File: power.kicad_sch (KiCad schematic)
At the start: 32 parts, among them J18 Conn_01x06, U32 LTC4121, U33 BQ25883RGER

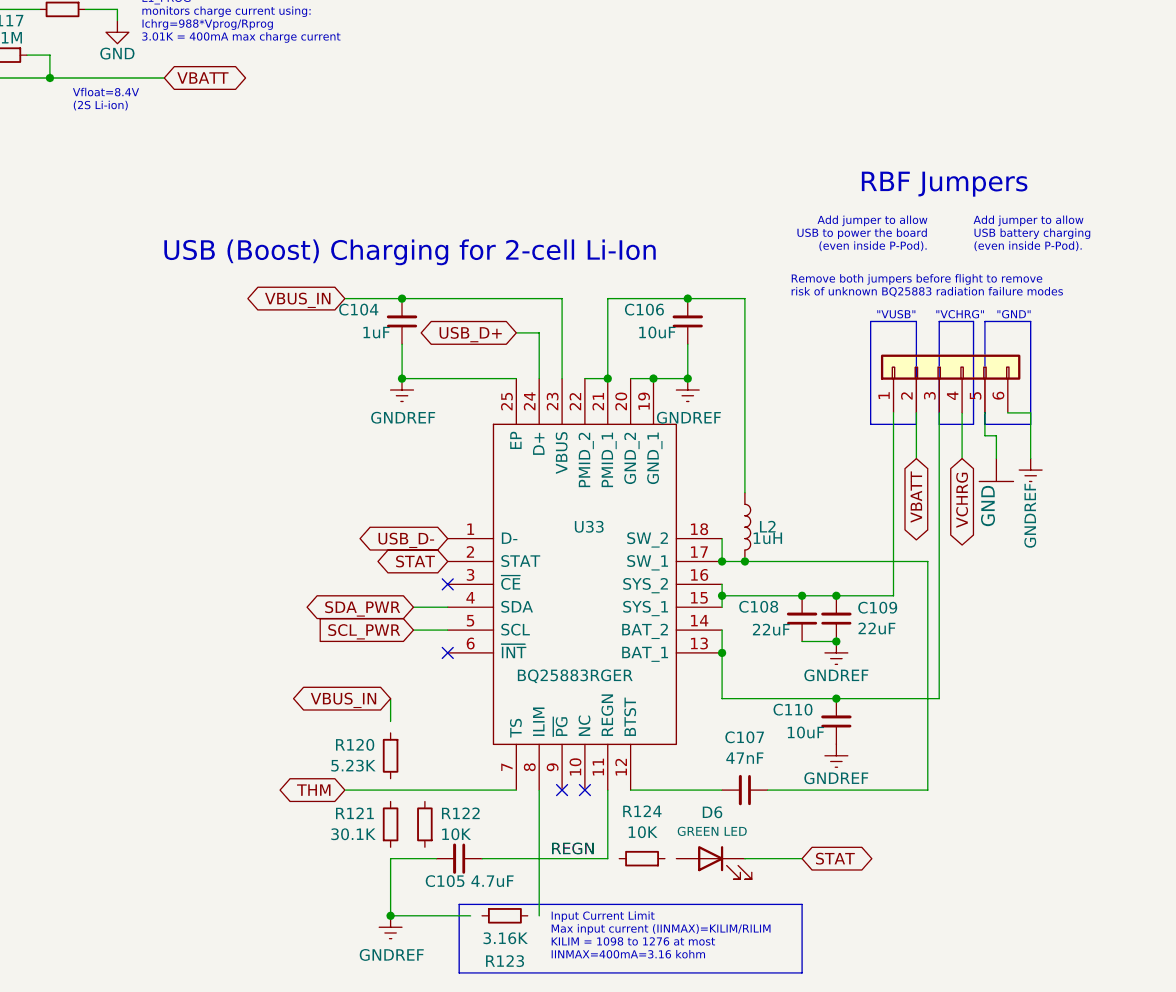
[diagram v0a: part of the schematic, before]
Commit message: Backup
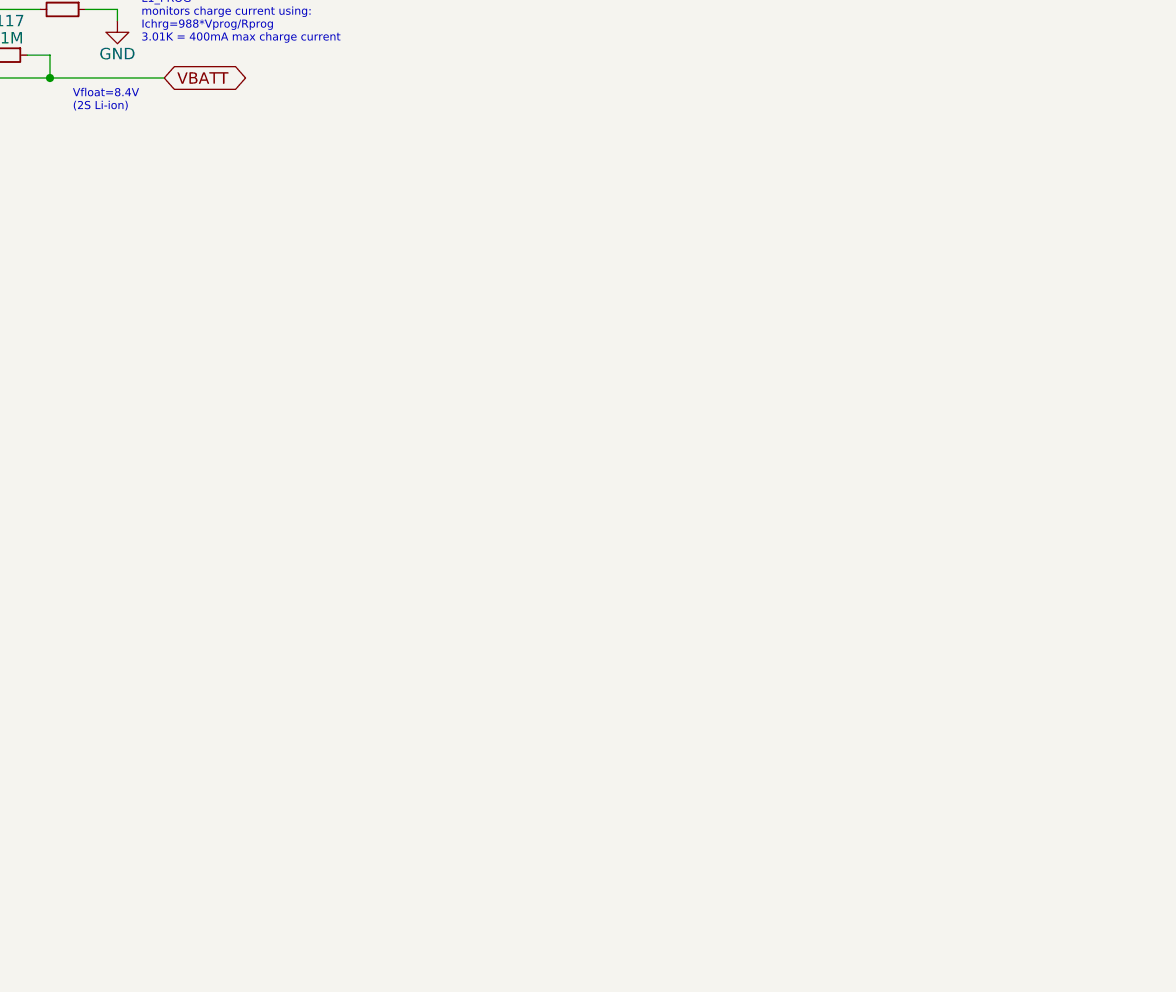
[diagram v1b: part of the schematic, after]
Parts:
- removed C104: 1uF, Capacitor_SMD:C_0603_1608Metric, symbol Device:C_Small
- removed C105: 4.7uF, Capacitor_SMD:C_0603_1608Metric, symbol Device:C_Small
- removed C106, C110: 10uF, Capacitor_SMD:C_0603_1608Metric, symbol Device:C_Small
- removed C107: 47nF, Capacitor_SMD:C_0603_1608Metric, symbol Device:C_Small
- removed C108, C109: 22uF, Capacitor_SMD:C_0603_1608Metric, symbol Device:C_Small
- removed D6: GREEN LED, LED_SMD:LED_0603_1608Metric, symbol Device:LED
- removed J18: Conn_01x06, Connector_PinHeader_2.54mm:PinHeader_1x06_P2.54mm_Vertical, symbol Connector_Generic:Conn_01x06
- removed L2: 1uH, mainboard:L_2510, symbol Device:L
- removed R120: 5.23K, Resistor_SMD:R_0603_1608Metric, symbol Device:R_Small
- removed R121: 30.1K, Resistor_SMD:R_0603_1608Metric, symbol Device:R_Small
- removed R122, R124: 10K, Resistor_SMD:R_0603_1608Metric, symbol Device:R_Small
- removed R123: 3.16K, Resistor_SMD:R_0603_1608Metric, symbol Device:R_Small
- removed U33: BQ25883RGER, mainboard:QFN50P400X400X100-25N-D, symbol mainboard:BQ25883RGER
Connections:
- no-connect marks 4 -> 0
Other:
- note removed: ""GND""
- note removed: ""VCHRG""
- note removed: ""VUSB""
- note removed: "Add jumper to allow USB battery charging (even inside P-Pod)."
- note removed: "Add jumper to allow USB to power the board (even inside P-Pod)."
- note removed: "Input Current Limit Max input current (IINMAX)=KILIM/RILIM KILIM = 1098 to 1276 at most IINMAX=400mA=3.16 kohm"
- note removed: "RBF Jumpers"
- note removed: "Remove both jumpers before flight to remove risk of unknown BQ25883 radiation failure modes"
- note removed: "USB (Boost) Charging for 2-cell Li-Ion"
